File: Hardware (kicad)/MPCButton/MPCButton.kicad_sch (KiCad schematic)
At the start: 5 parts, among them P1 62100421921

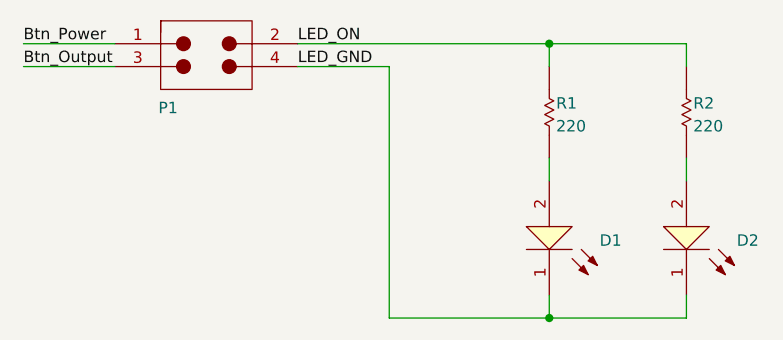
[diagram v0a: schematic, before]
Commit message: fix kicad projects
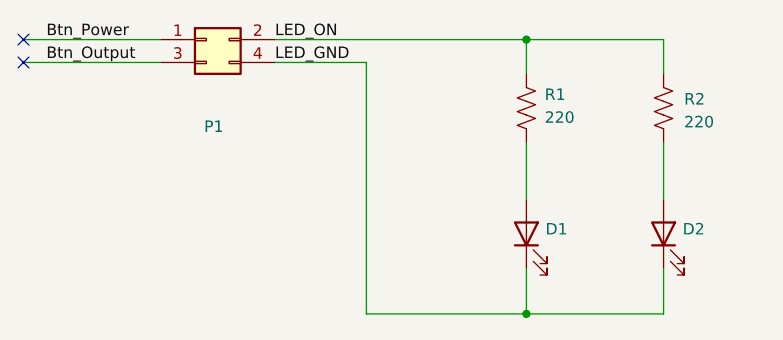
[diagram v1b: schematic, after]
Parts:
- D1, D2: footprint WL-SMCC_0603_150060xx73220 -> Wurth_WL-SMCW (rev24b):WL-SMCW_0603_150060xx75000; symbol Altium_WL-SMCC (rev24a):root_3_150060RS73220_Altium_WL-SMCC (rev24a).IntLib -> Device:LED
- P1: footprint 62100421921 -> Wurth_WR-PHD (rev24a):62100421921; symbol Wurth_WR-PHD (rev24a):root_0_62100421921_Wurth_WR-PHD (rev24a).IntLib -> Connector_Generic:Conn_02x02_Odd_Even
- R1, R2: footprint RESC0603(1608)_N -> Resistor_SMD:R_0603_1608Metric_Pad0.98x0.95mm_HandSolder; symbol Passive SMD:root_1_RES_Passive SMD.IntLib -> Device:R_US
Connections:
- no-connect marks 0 -> 2
